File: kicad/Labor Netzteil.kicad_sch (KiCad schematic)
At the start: 35 parts, among them J1 Fan, J10 Sec 1 a, J11 Sec 2 a, J12 Sec 2 b, J13 Sec 2 c, J14 Sec 2 d, J15 Out_2_02, J16 Out_2_01, J17 Out_1, J18 Out_2, J19 NeoPixel, J2 OLED, J3 +5V In, J4 GND 5V In, J5 Out_1_01, J6 Out_1_02, J7 Sec 1 d, J8 Sec 1 c, J9 Sec 1 b, U1 2-Relais-Modul, U2 ESP32-DevKitC, U3 74HC245, U4 DS18B20

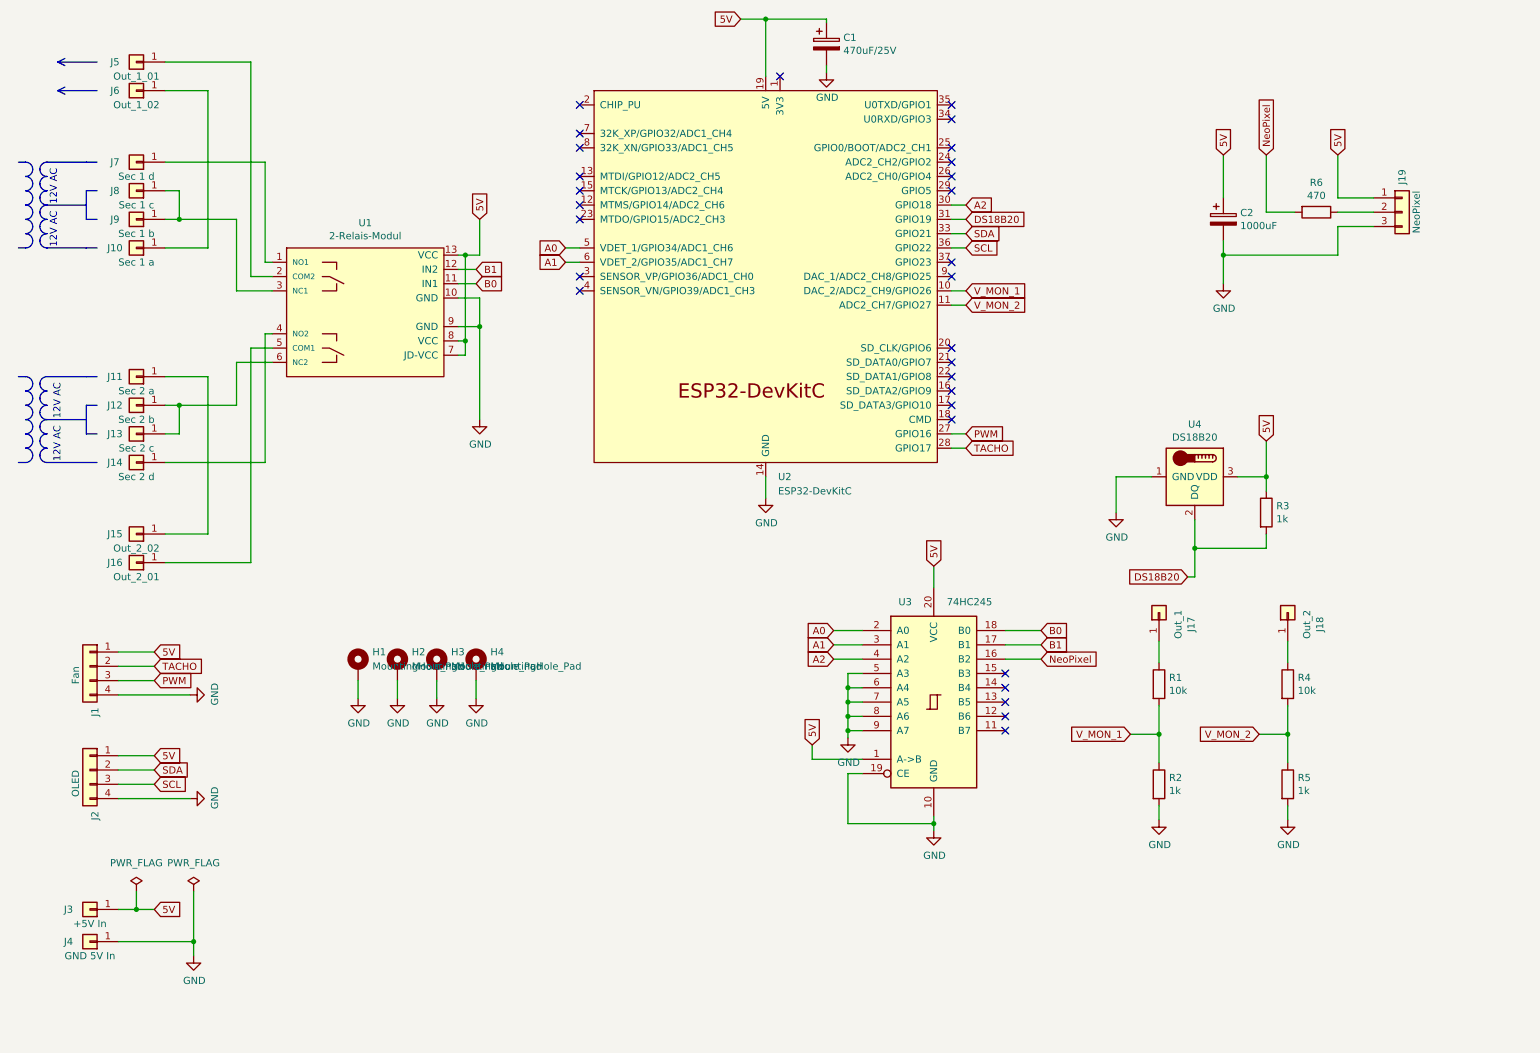
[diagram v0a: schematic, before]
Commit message: Grundlegende Änderung der Schaltung, siehe README
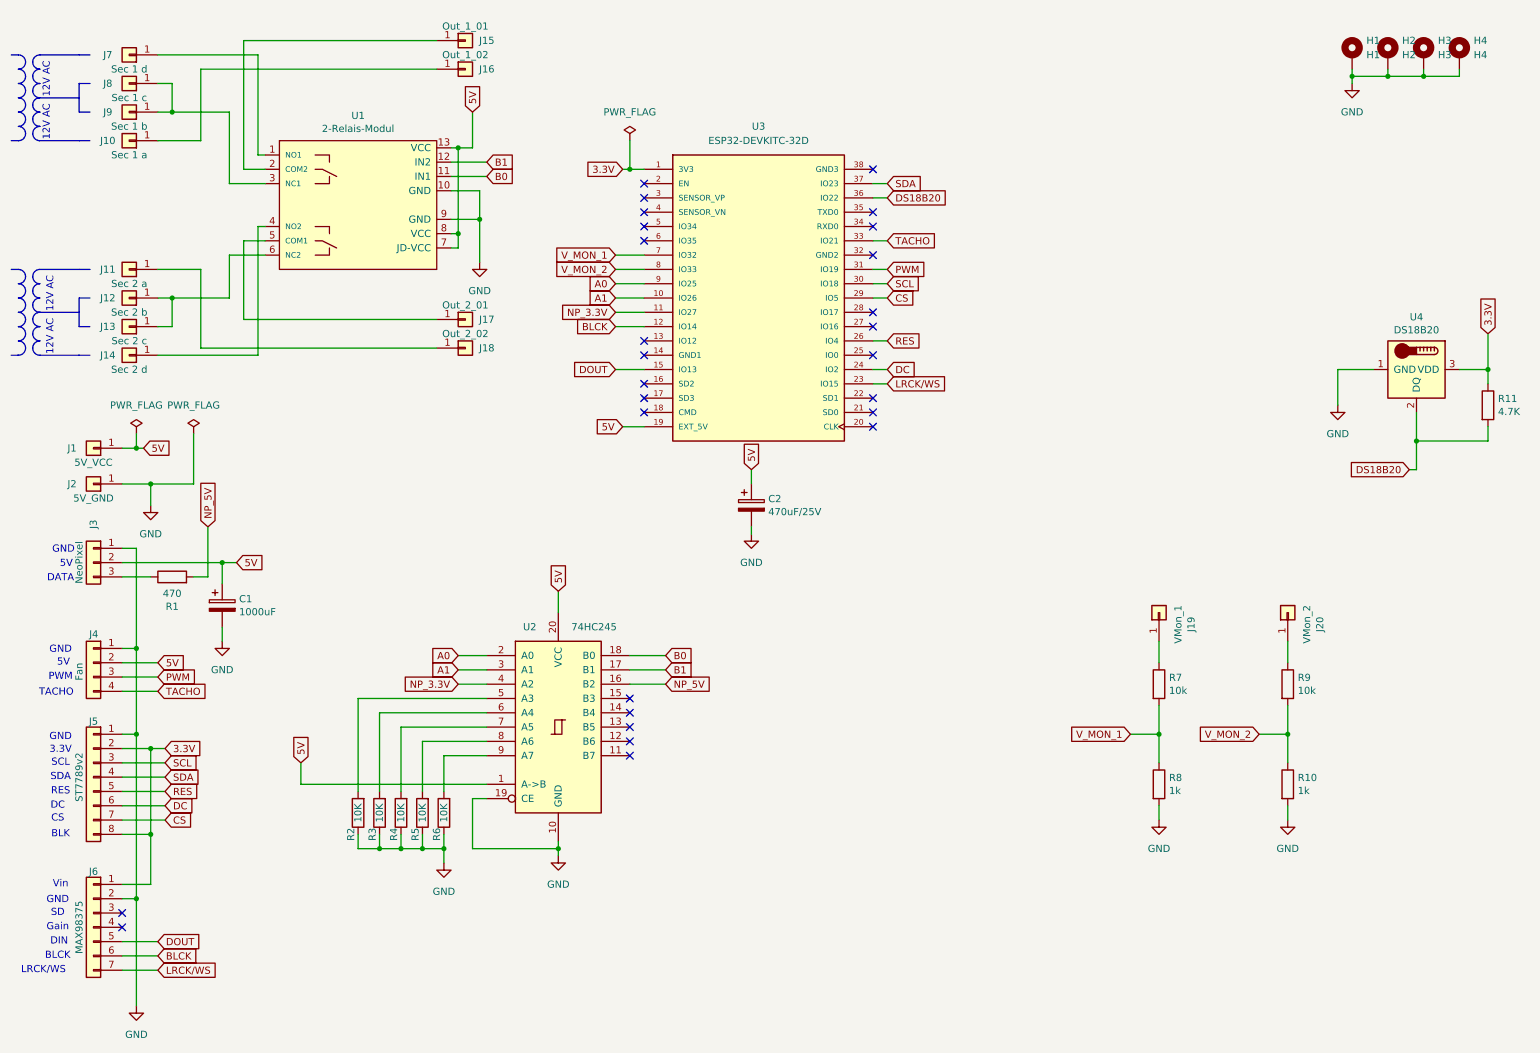
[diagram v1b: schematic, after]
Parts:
- removed J2: OLED, Connector_JST:JST_XH_B4B-XH-A_1x04_P2.50mm_Vertical, symbol Connector_Generic:Conn_01x04
- removed J3: +5V In, Connector_Pin:Pin_D1.3mm_L11.0mm_LooseFit, symbol Connector_Generic:Conn_01x01
- removed J4: GND 5V In, Connector_Pin:Pin_D1.3mm_L11.0mm_LooseFit, symbol Connector_Generic:Conn_01x01
- removed U2: ESP32-DevKitC, PCM_Espressif:ESP32-DevKitC, symbol PCM_Espressif:ESP32-DevKitC
- added J1: 5V_VCC, Connector_Pin:Pin_D1.3mm_L11.0mm_LooseFit, symbol Connector_Generic:Conn_01x01
- added J2: 5V_GND, Connector_Pin:Pin_D1.3mm_L11.0mm_LooseFit, symbol Connector_Generic:Conn_01x01
- added J5: ST7789v2, Connector_JST:JST_XH_B8B-XH-A_1x08_P2.50mm_Vertical, symbol Connector_Generic:Conn_01x08
- added J6: MAX98375, Connector_JST:JST_XH_B7B-XH-A_1x07_P2.50mm_Vertical, symbol Connector_Generic:Conn_01x07
- added R2, R3, R4, R5, R6: 10K, Resistor_THT:R_Axial_DIN0204_L3.6mm_D1.6mm_P7.62mm_Horizontal, symbol Device:R
- added U3: ESP32-DEVKITC-32D, RF_Module:ESP32-DevKitC-V4-b, symbol MCU_Espressif:ESP32-DEVKITC-32D
- C1: renamed from C2; footprint Capacitor_THT:CP_Radial_D14.0mm_P5.00mm -> Capacitor_THT:CP_Radial_D8.0mm_P5.00mm
- C2: renamed from C1; footprint MountingHole:MountingHole_3.2mm_M3_DIN965_Pad -> Capacitor_THT:CP_Radial_D8.0mm_P3.50mm
- H1: value MountingHole_Pad -> H1; footprint MountingHole:MountingHole_3.2mm_M3_ISO14580_Pad -> MountingHole:MountingHole_3.2mm_M3_Pad_Via
- H2: value MountingHole_Pad -> H2; footprint MountingHole:MountingHole_3.2mm_M3_ISO14580_Pad -> MountingHole:MountingHole_3.2mm_M3_Pad_Via
- H3: value MountingHole_Pad -> H3; footprint MountingHole:MountingHole_3.2mm_M3_ISO14580_Pad -> MountingHole:MountingHole_3.2mm_M3_Pad_Via
- H4: value MountingHole_Pad -> H4; footprint MountingHole:MountingHole_3.2mm_M3_ISO14580_Pad -> MountingHole:MountingHole_3.2mm_M3_Pad_Via
- J19: renamed from J17; value Out_1 -> VMon_1; footprint Connector_Pin:Pin_D1.0mm_L10.0mm -> Connector_PinHeader_1.00mm:PinHeader_1x01_P1.00mm_Vertical
- J20: renamed from J18; value Out_2 -> VMon_2; footprint Connector_Pin:Pin_D1.0mm_L10.0mm -> Connector_PinHeader_1.00mm:PinHeader_1x01_P1.00mm_Vertical
- R1: renamed from R6; footprint Resistor_THT:R_Axial_DIN0207_L6.3mm_D2.5mm_P10.16mm_Horizontal -> Resistor_THT:R_Axial_DIN0204_L3.6mm_D1.6mm_P7.62mm_Horizontal
- R10: renamed from R5; footprint Resistor_THT:R_Axial_DIN0207_L6.3mm_D2.5mm_P10.16mm_Horizontal -> Resistor_THT:R_Axial_DIN0204_L3.6mm_D1.6mm_P7.62mm_Horizontal
- R11: renamed from R3; value 1k -> 4.7K; footprint Resistor_THT:R_Axial_DIN0207_L6.3mm_D2.5mm_P10.16mm_Horizontal -> Resistor_THT:R_Axial_DIN0204_L3.6mm_D1.6mm_P7.62mm_Horizontal
- R7: renamed from R1; footprint Resistor_THT:R_Axial_DIN0207_L6.3mm_D2.5mm_P10.16mm_Horizontal -> Resistor_THT:R_Axial_DIN0204_L3.6mm_D1.6mm_P7.62mm_Horizontal
- R8: renamed from R2; footprint Resistor_THT:R_Axial_DIN0207_L6.3mm_D2.5mm_P10.16mm_Horizontal -> Resistor_THT:R_Axial_DIN0204_L3.6mm_D1.6mm_P7.62mm_Horizontal
- R9: renamed from R4; footprint Resistor_THT:R_Axial_DIN0207_L6.3mm_D2.5mm_P10.16mm_Horizontal -> Resistor_THT:R_Axial_DIN0204_L3.6mm_D1.6mm_P7.62mm_Horizontal
- renumbered J5 to J15, J6 to J16, J16 to J17, J15 to J18, J19 to J3, J1 to J4, U3 to U2
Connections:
- net 5V: now also J3.2 (Pin_2), J4.2 (Pin_2), J1.1 (Pin_1), U3.19 (EXT_5V); no longer J3.1 (Pin_1), J4.1 (Pin_1), R11.1, U4.3 (VDD)
- net A0: now also U3.9 (IO25)
- net A1: now also U3.10 (IO26)
- net DS18B20: now also U3.36 (IO22)
- net GND: now also J3.1 (Pin_1), J4.1 (Pin_1), J2.1 (Pin_1), J5.1 (Pin_1), J6.2 (Pin_2), R2.1, R3.1, R4.1, R5.1, R6.1; no longer J3.3 (Pin_3), J4.4 (Pin_4), U2.5 (A3), U2.6 (A4), U2.7 (A5), U2.8 (A6), U2.9 (A7)
- net PWM: now also U3.31 (IO19)
- net SCL: now also J5.3 (Pin_3), U3.30 (IO18)
- net SDA: now also J5.4 (Pin_4), U3.37 (IO23)
- net TACHO: now also J4.4 (Pin_4), U3.33 (IO21); no longer J4.2 (Pin_2)
- net V_MON_1: now also U3.7 (IO32)
- net V_MON_2: now also U3.8 (IO33)
- net at R1.1: now also J3.3 (Pin_3); no longer J3.2 (Pin_2)
- net A2 renamed NP_3.3V
- net NP_3.3V: now also U3.11 (IO27)
- net NeoPixel renamed NP_5V
- new net: R2.2, U2.5 (A3)
- new net: R3.2, U2.6 (A4)
- new net: R4.2, U2.7 (A5)
- new net: R5.2, U2.8 (A6)
- new net: R6.2, U2.9 (A7)
- new net 3.3V: J5.2 (Pin_2), J5.8 (Pin_8), J6.1 (Pin_1), R11.1, U3.1 (3V3), U4.3 (VDD)
- new net BLCK: J6.6 (Pin_6), U3.12 (IO14)
- new net CS: J5.7 (Pin_7), U3.29 (IO5)
- new net DC: J5.6 (Pin_6), U3.24 (IO2)
- new net DOUT: J6.5 (Pin_5), U3.15 (IO13)
- new net LRCK/WS: J6.7 (Pin_7), U3.23 (IO15)
- new net RES: J5.5 (Pin_5), U3.26 (IO4)
- no-connect marks 29 -> 27
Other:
- note added: "3.3V"
- note added: "5V"
- note added: "BLCK"
- note added: "BLK"
- note added: "CS"
- note added: "DATA"
- note added: "DC"
- note added: "DIN"
- note added: "GND"
- note added: "Gain"
- note added: "LRCK/WS"
- note added: "PWM"
- note added: "RES"
- note added: "SCL"
- note added: "SD"
- note added: "SDA"
- note added: "TACHO"
- note added: "Vin"
- moved on the sheet: C1, C2, H1, H2, H3, H4, J10, J11, J12, J13, J14, J15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
